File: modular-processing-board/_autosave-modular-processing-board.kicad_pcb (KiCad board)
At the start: 6 copper layers, 90 x 90 mm, 159 parts, among them J202 Conn_02x06_Odd_Even, J401 Micro_SD_Card, J501 Plug_Hirose_DF40_2x40_DF40C-8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, J502 Conn_02x06_Odd_Even, J601 Conn_Coaxial_Small, J604 Conn_Coaxial_Small, J701 Conn_02x02_Odd_Even, J801 TYPE-C-31-M-12, SW201 SW_Push, SW602 SW_Push, U1002 THS4521IDGK, U201 STM32H723ZGTx, U301 W9825G6KH-6, U302 W9825G6KH-6, U401 SRV05-4, U601 LMV321, U602 TL432DBZ, U603 THS4521IDGK, U701 AMS1117-3.3, Y1201 25MHz

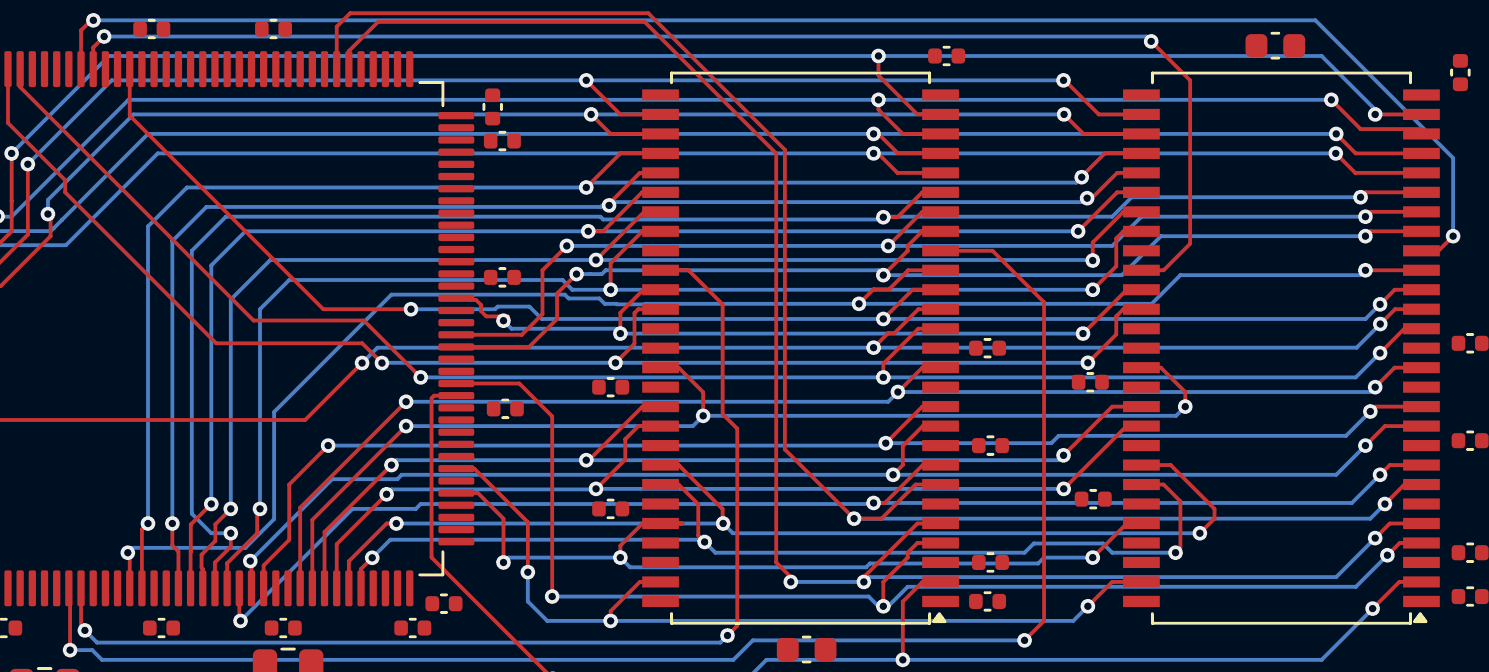
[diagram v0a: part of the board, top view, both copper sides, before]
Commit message: figuring out delay matching for sdram
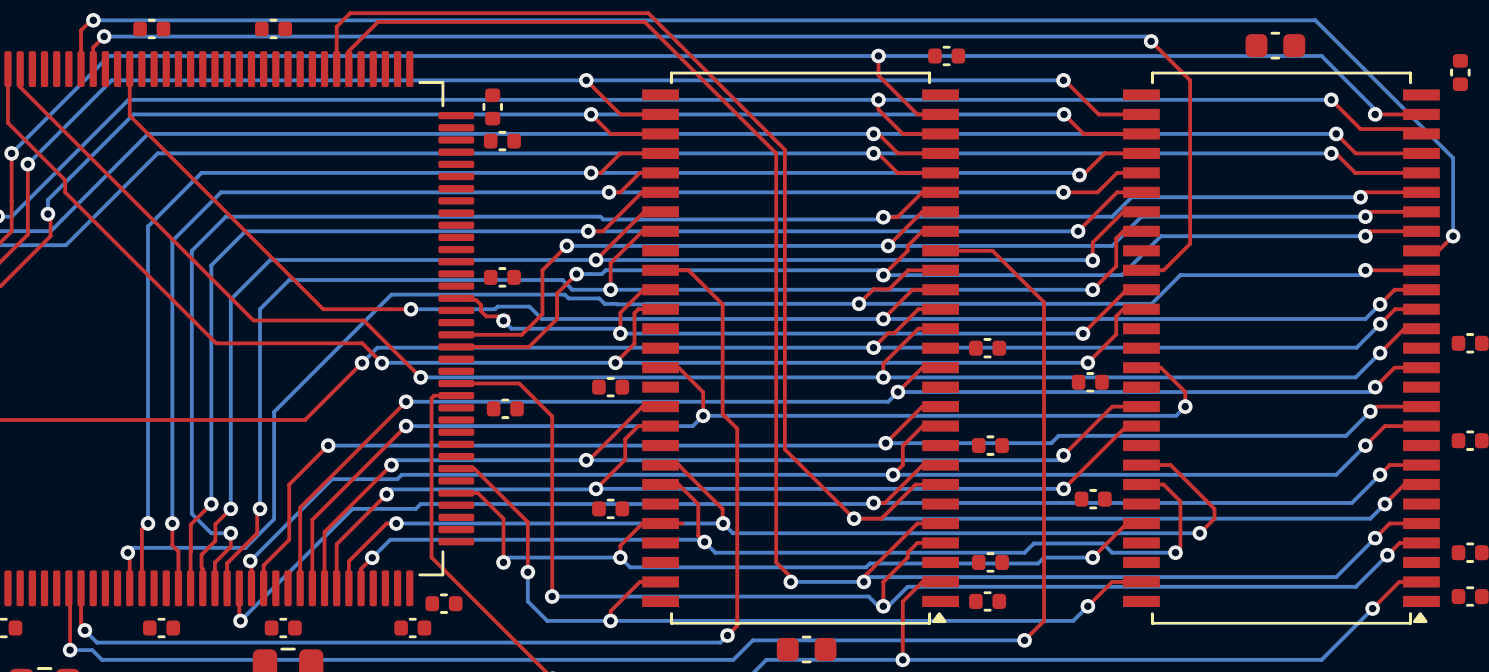
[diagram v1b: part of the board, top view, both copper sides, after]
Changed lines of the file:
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@@
+	)
+	(segment
+		(start 119.8 80.6)
+		(end 120.6 80.6)
+		(width 0.1565)
+		(layer "F.Cu")
+		(net 120)
+	)
+	(segment
+		(start 119 81.4)
+		(end 119.8 80.6)
+		(width 0.1565)
+		(layer "F.Cu")
+		(net 120)
+	)
+	(segment
+		(start 81.25 96.15)
+		(end 81.25 97.6625)
+		(width 0.1565)
+		(layer "F.Cu")
+		(net 120)
+	)
+	(segment
+		(start 81 95)
+		(end 81 95.9)
+		(width 0.1565)
+		(layer "F.Cu")
+		(net 120)
+	)
+	(segment
+		(start 81 95.9)
+		(end 81.25 96.15)
+		(width 0.1565)
+		(layer "F.Cu")
+		(net 120)
 	)
 	(segment
@@
 	)
 	(segment
-		(start 98.935678 81.935678)
-		(end 98.935678 81.864322)
+		(start 117.6 81.4)
+		(end 119 81.4)
 		(width 0.1565)
 		(layer "F.Cu")
@@
 	)
 	(segment
-		(start 118.76054 81.63946)
-		(end 119.8 80.6)
+		(start 99.4 81.4)
+		(end 100.2 80.6)
 		(width 0.1565)
 		(layer "F.Cu")
@@
 	)
 	(segment
-		(start 81.25 96.15)
-		(end 81.25 97.6625)
+		(start 98.935678 81.4)
+		(end 99.4 81.4)
 		(width 0.1565)
 		(layer "F.Cu")
 		(net 120)
 	)
-	(segment
-		(start 119.8 80.6)
-		(end 120.6 80.6)
-		(width 0.1565)
-		(layer "F.Cu")
+	(via
+		(at 98.935678 81.4)
+		(size 0.6)
+		(drill 0.3)
+		(layers "F.Cu" "B.Cu")
 		(net 120)
 	)
-	(segment
-		(start 81 95)
-		(end 81 95.9)
-		(width 0.1565)
-		(layer "F.Cu")
+	(via
+		(at 117.6 81.4)
+		(size 0.6)
+		(drill 0.3)
+		(layers "F.Cu" "B.Cu")
 		(net 120)
 	)
-	(segment
-		(start 81 95.9)
-		(end 81.25 96.15)
-		(width 0.1565)
-		(layer "F.Cu")
+	(via
+		(at 81 95)
+		(size 0.6)
+		(drill 0.3)
+		(layers "F.Cu" "B.Cu")
 		(net 120)
 	)
 	(segment
-		(start 98.935678 81.864322)
-		(end 100.2 80.6)
-		(width 0.1565)
-		(layer "F.Cu")
+		(start 98.935678 81.4)
+		(end 83 81.4)
+		(width 0.1565)
+		(layer "B.Cu")
 		(net 120)
 	)
 	(segment
-		(start 118.569733 81.63946)
-		(end 118.76054 81.63946)
-		(width 0.1565)
-		(layer "F.Cu")
+		(start 83 81.4)
+		(end 81 83.4)
+		(width 0.1565)
+		(layer "B.Cu")
 		(net 120)
 	)
-	(via
-		(at 98.935678 81.935678)
-		(size 0.6)
-		(drill 0.3)
-		(layers "F.Cu" "B.Cu")
+	(segment
+		(start 81 83.4)
+		(end 81 95)
+		(width 0.1565)
+		(layer "B.Cu")
 		(net 120)
 	)
-	(via
-		(at 118.569733 81.63946)
-		(size 0.6)
-		(drill 0.3)
-		(layers "F.Cu" "B.Cu")
-		(net 120)
-	)
-	(via
-		(at 81 95)
-		(size 0.6)
-		(drill 0.3)
-		(layers "F.Cu" "B.Cu")
-		(net 120)
-	)
-	(segment
-		(start 82.4 82)
-		(end 98.6 82)
-		(width 0.1565)
-		(layer "B.Cu")
-		(net 120)
-	)
-	(segment
-		(start 81 95)
-		(end 81 83.4)
-		(width 0.1565)
-		(layer "B.Cu")
-		(net 120)
-	)
-	(segment
-		(start 118.409193 81.8)
-		(end 118.569733 81.63946)
-		(width 0.1565)
-		(layer "B.Cu")
-		(net 120)
-	)
-	(segment
-		(start 98.6 82)
-		(end 98.664322 81.935678)
-		(width 0.1565)
-		(layer "B.Cu")
-		(net 120)
-	)
-	(segment
-		(start 81 83.4)
-		(end 82.4 82)
-		(width 0.1565)
-		(layer "B.Cu")
-		(net 120)
-	)
-	(segment
-		(start 98.664322 81.935678)
-		(end 98.935678 81.935678)
-		(width 0.1565)
-		(layer "B.Cu")
-		(net 120)
-	)
-	(segment
-		(start 98.935678 81.935678)
-		(end 99.071356 81.8)
-		(width 0.1565)
-		(layer "B.Cu")
-		(net 120)
-	)
-	(segment
-		(start 99.071356 81.8)
-		(end 118.409193 81.8)
+	(segment
+		(start 98.935678 81.4)
+		(end 117.6 81.4)
 		(width 0.1565)
 		(layer "B.Cu")
@@
 	)
 	(segment
+		(start 129.582231 80.6)
+		(end 132.1 80.6)
+		(width 0.1565)
+		(layer "F.Cu")
+		(net 149)
+	)
+	(segment
 		(start 109.8 79.8)
 		(end 109.982231 79.8)
@@
 	)
 	(segment
-		(start 129.582231 80.6)
-		(end 132.1 80.6)
+		(start 128.6 79.8)
+		(end 128.782231 79.8)
 		(width 0.1565)
 		(layer "F.Cu")
@@
 	)
 	(via
-		(at 128.782231 79.8)
+		(at 128.6 79.8)
 		(size 0.6)
 		(drill 0.3)
@@
 	)
 	(segment
-		(start 128.782231 79.8)
-		(end 109.8 79.8)
-		(width 0.1565)
-		(layer "B.Cu")
-		(net 149)
-	)
-	(segment
 		(start 80.4 79.8)
 		(end 76.629635 83.570365)
@@
 	)
 	(segment
+		(start 128.6 79.8)
+		(end 109.8 79.8)
+		(width 0.1565)
+		(layer "B.Cu")
+		(net 149)
+	)
+	(segment
 		(start 111.8 81.4)
 		(end 112.55 81.4)
@@
 	)
 	(segment
+		(start 118.347156 80.747156)
+		(end 119.294312 79.8)
+		(width 0.1565)
+		(layer "F.Cu")
+		(net 151)
+	)
+	(segment
+		(start 99.4 79.8)
+		(end 101.05 79.8)
+		(width 0.1565)
+		(layer "F.Cu")
+		(net 151)
+	)
+	(segment
 		(start 79.75 97.6625)
 		(end 79.75 95.25)
@@
 	)
 	(segment
-		(start 118.347156 80.77825)
-		(end 118.347156 80.747156)
+		(start 118.258031 80.689125)
+		(end 118.316062 80.747156)
 		(width 0.1565)
 		(layer "F.Cu")
@@
 	)
 	(segment
-		(start 99.4 79.8)
-		(end 101.05 79.8)
-		(width 0.1565)
-		(layer "F.Cu")
-		(net 151)
-	)
-	(segment
-		(start 118.347156 80.747156)
-		(end 119.294312 79.8)
+		(start 98.2 80.6)
+		(end 98.6 80.6)
 		(width 0.1565)
 		(layer "F.Cu")
@@
 	)
 	(segment
-		(start 98 81.2)
+		(start 98.6 80.6)
 		(end 99.4 79.8)
+		(width 0.1565)
+		(layer "F.Cu")
+		(net 151)
+	)
+	(segment
+		(start 118.316062 80.747156)
+		(end 118.347156 80.747156)
 		(width 0.1565)
 		(layer "F.Cu")
@@
 	)
 	(via
-		(at 98 81.2)
+		(at 98.2 80.6)
 		(size 0.6)
 		(drill 0.3)
@@
 	)
 	(via
-		(at 118.347156 80.77825)
+		(at 118.258031 80.689125)
 		(size 0.6)
 		(drill 0.3)
@@
 	)
 	(segment
-		(start 98.2 81)
-		(end 98 81.2)
+		(start 80 82.8)
+		(end 80 95)
 		(width 0.1565)
 		(layer "B.Cu")
@@
 	)
 	(segment
-		(start 80 82.8)
-		(end 81.6 81.2)
+		(start 98.2 80.6)
+		(end 82.2 80.6)
 		(width 0.1565)
 		(layer "B.Cu")
@@
 	)
 	(segment
-		(start 118.125406 81)
-		(end 98.2 81)
+		(start 118.168906 80.6)
+		(end 98.2 80.6)
 		(width 0.1565)
 		(layer "B.Cu")
@@
 	)
 	(segment
-		(start 80 95)
+		(start 118.258031 80.689125)
+		(end 118.168906 80.6)
+		(width 0.1565)
+		(layer "B.Cu")
+		(net 151)
+	)
+	(segment
+		(start 82.2 80.6)
 		(end 80 82.8)
 		(width 0.1565)
 		(layer "B.Cu")
-		(net 151)
-	)
-	(segment
-		(start 118.347156 80.77825)
-		(end 118.125406 81)
-		(width 0.1565)
-		(layer "B.Cu")
-		(net 151)
-	)
-	(segment
-		(start 81.6 81.2)
-		(end 98 81.2)
-		(width 0.1565)
-		(layer "B.Cu")
